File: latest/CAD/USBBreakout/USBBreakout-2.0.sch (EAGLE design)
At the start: 31 parts, among them IC1 MIC5203-3.3YM5-TR, J1 OSTVN02A150, J2 10118194-0001LF, J3 RJ-82A86MMNL, Q1 DMP3099L-7, Q2 DMP3099L-7, Q3 DMP3099L-7, Q4 BSS138

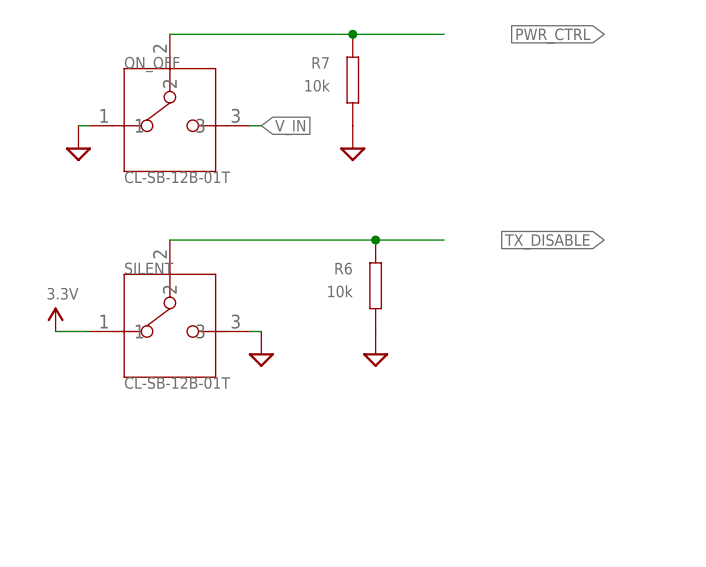
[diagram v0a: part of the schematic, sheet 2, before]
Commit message: Updated CAD
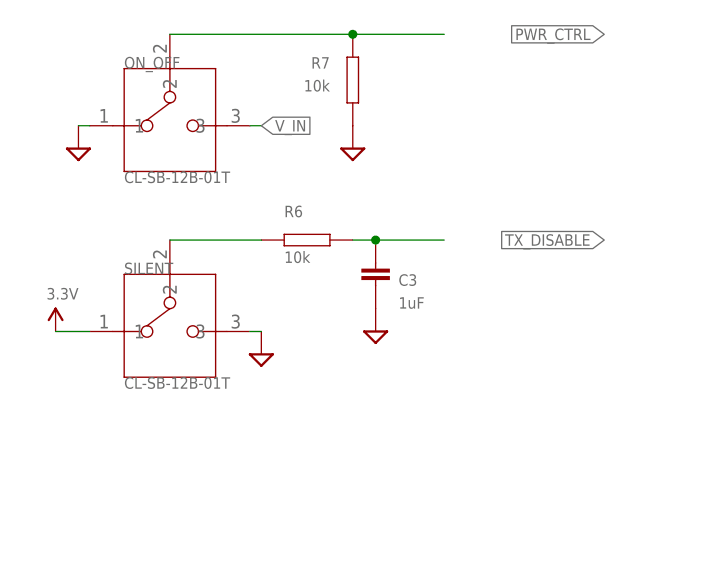
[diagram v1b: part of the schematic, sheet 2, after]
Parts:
- added C3: 1uF, MyPassives:CAPACITOR0603
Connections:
- new net N$5: R6.P$1, SILENT.2
- net GND: now also C3.2; no longer R6.P$2
- net TX_DISABLE: now also C3.1, R6.P$2; no longer R6.P$1, SILENT.2
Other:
- moved on the sheet: R6
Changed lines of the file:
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@@
 <part name="R7" library="MyPassives" deviceset="RESISTOR" device="0603" value="10k"/>
 <part name="SUPPLY26" library="supply2" deviceset="GND" device=""/>
+<part name="SUPPLY9" library="supply2" deviceset="GND" device=""/>
 <part name="R6" library="MyPassives" deviceset="RESISTOR" device="0603" value="10k"/>
-<part name="SUPPLY27" library="supply2" deviceset="GND" device=""/>
-<part name="SUPPLY9" library="supply2" deviceset="GND" device=""/>
+<part name="C3" library="MyPassives" deviceset="CAPACITOR" device="0603" value="1uF"/>
+<part name="SUPPLY14" library="supply2" deviceset="GND" device=""/>
 </parts>
 <sheets>
@@
 </instance>
 <instance part="SUPPLY26" gate="GND" x="71.12" y="121.92" smashed="yes" rot="MR0"/>
-<instance part="R6" gate="G$1" x="73.66" y="106.68" smashed="yes" rot="R270">
-<attribute name="NAME" x="71.12" y="109.22" size="1.27" layer="95" rot="R180"/>
-<attribute name="VALUE" x="71.12" y="106.68" size="1.27" layer="96" rot="R180"/>
-</instance>
-<instance part="SUPPLY27" gate="GND" x="73.66" y="99.06" smashed="yes" rot="MR0"/>
 <instance part="SUPPLY9" gate="GND" x="60.96" y="99.06" smashed="yes" rot="MR0"/>
+<instance part="R6" gate="G$1" x="66.04" y="111.76" smashed="yes">
+<attribute name="NAME" x="63.5" y="114.3" size="1.27" layer="95"/>
+<attribute name="VALUE" x="63.5" y="109.22" size="1.27" layer="96"/>
+</instance>
+<instance part="C3" gate="G$1" x="73.66" y="109.22" smashed="yes">
+<attribute name="NAME" x="76.2" y="106.68" size="1.27" layer="95"/>
+<attribute name="VALUE" x="76.2" y="104.14" size="1.27" layer="96"/>
+</instance>
+<instance part="SUPPLY14" gate="GND" x="73.66" y="101.6" smashed="yes" rot="MR0"/>
 </instances>
 <busses>
@@
 </segment>
 <segment>
-<pinref part="R6" gate="G$1" pin="P$2"/>
-<pinref part="SUPPLY27" gate="GND" pin="GND"/>
-</segment>
-<segment>
 <pinref part="SILENT" gate="A" pin="3"/>
 <pinref part="SUPPLY9" gate="GND" pin="GND"/>
 <wire x1="59.69" y1="101.6" x2="60.96" y2="101.6" width="0.1524" layer="91"/>
+</segment>
+<segment>
+<pinref part="C3" gate="G$1" pin="2"/>
+<pinref part="SUPPLY14" gate="GND" pin="GND"/>
 </segment>
 </net>
@@
 </segment>
 <segment>
-<pinref part="SILENT" gate="A" pin="2"/>
-<wire x1="50.8" y1="111.76" x2="73.66" y2="111.76" width="0.1524" layer="91"/>
-<pinref part="R6" gate="G$1" pin="P$1"/>
+<wire x1="71.12" y1="111.76" x2="73.66" y2="111.76" width="0.1524" layer="91"/>
+<label x="99.06" y="111.76" size="1.27" layer="95" rot="R180" xref="yes"/>
+<pinref part="R6" gate="G$1" pin="P$2"/>
+<pinref part="C3" gate="G$1" pin="1"/>
 <wire x1="73.66" y1="111.76" x2="81.28" y2="111.76" width="0.1524" layer="91"/>
 <junction x="73.66" y="111.76"/>
-<label x="99.06" y="111.76" size="1.27" layer="95" rot="R180" xref="yes"/>
 </segment>
 </net>
@@
 </segment>
 </net>
+<net name="N$5" class="0">
+<segment>
+<pinref part="SILENT" gate="A" pin="2"/>
+<wire x1="50.8" y1="111.76" x2="60.96" y2="111.76" width="0.1524" layer="91"/>
+<pinref part="R6" gate="G$1" pin="P$1"/>
+</segment>
+</net>
